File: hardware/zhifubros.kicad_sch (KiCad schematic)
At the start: 7 parts, among them J1 Conn_01x09, U1 XIAO-ESP32-C3-SMD, U2 GY-521, U3 GY-521

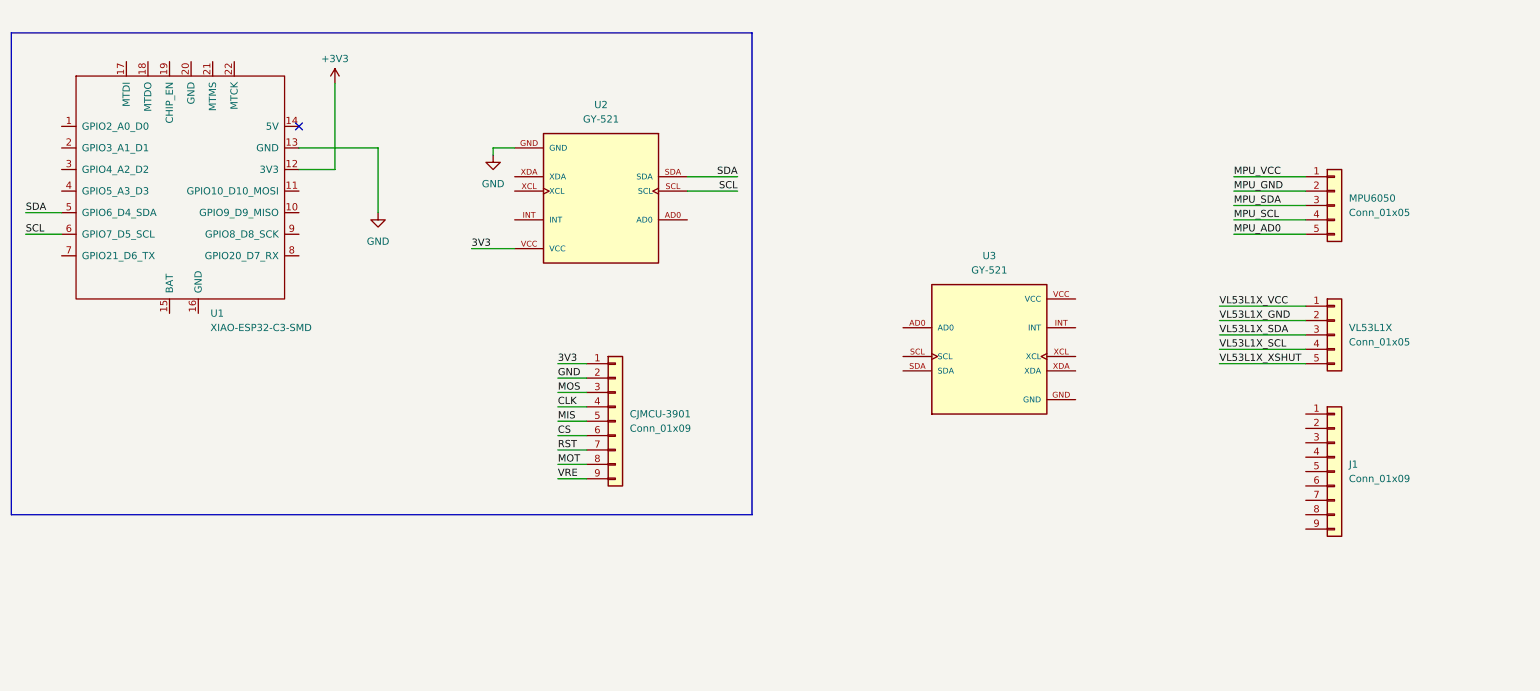
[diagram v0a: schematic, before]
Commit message: fix: schema
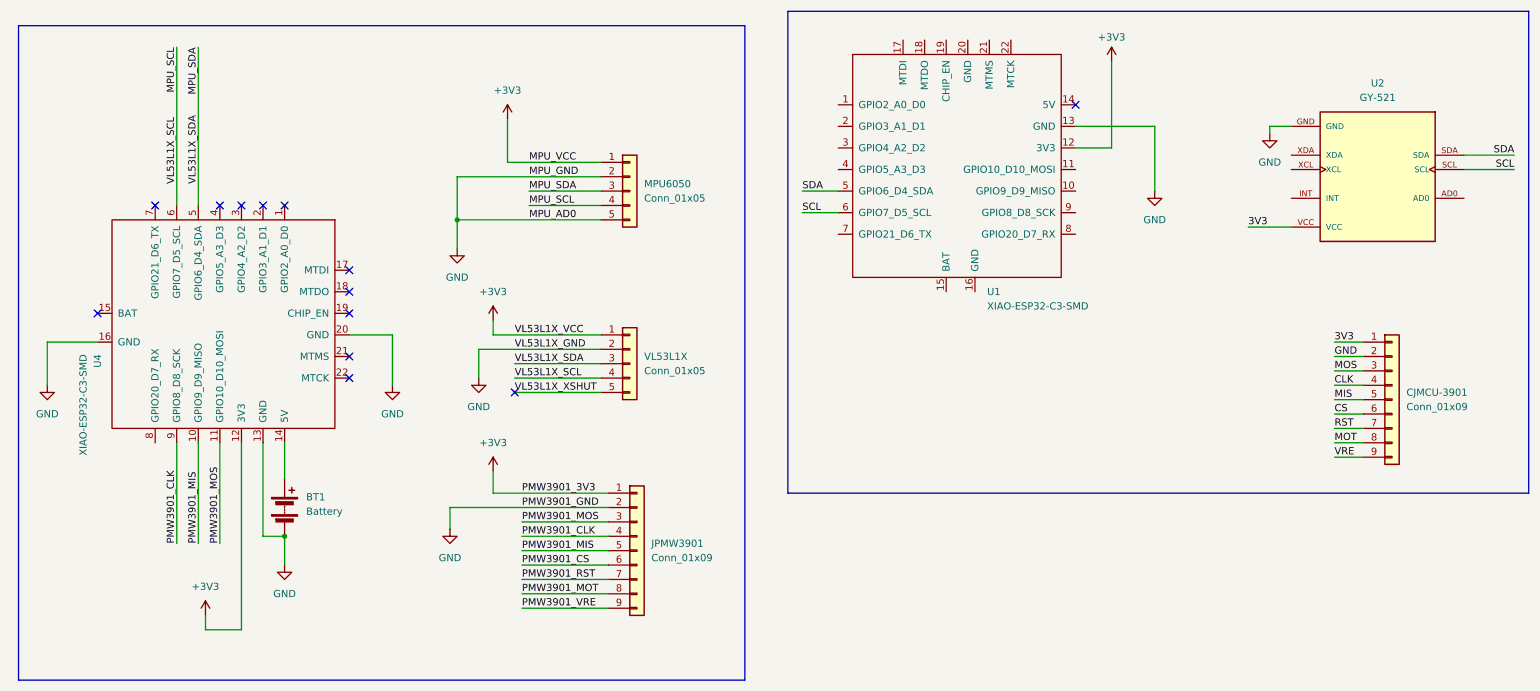
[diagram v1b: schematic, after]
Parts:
- removed U3: GY-521, GY-521:MODULE_GY-521, symbol mpu:GY-521
- added BT1: Battery, symbol Device:Battery
- added U4: XIAO-ESP32-C3-SMD, symbol xiao:XIAO-ESP32-C3-SMD
- renumbered J1 to JPMW3901
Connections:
- net MPU_AD0 is gone; now on net GND: MPU6050.5 (Pin_5)
- net MPU_GND is gone; now on net GND: MPU6050.2 (Pin_2)
- net MPU_VCC is gone; now on net +3V3: MPU6050.1 (Pin_1)
- net VL53L1X_GND is gone; now on net GND: VL53L1X.2 (Pin_2)
- net VL53L1X_SCL is gone; now on net MPU_SCL: VL53L1X.4 (Pin_4)
- net VL53L1X_SDA is gone; now on net MPU_SDA: VL53L1X.3 (Pin_3)
- net VL53L1X_VCC is gone; now on net +3V3: VL53L1X.1 (Pin_1)
- net +3V3: now also JPMW3901.1 (Pin_1), U4.12 (3V3)
- net GND: now also JPMW3901.2 (Pin_2), BT1.2 (-), U4.13 (GND), U4.16 (GND), U4.20 (GND)
- net MPU_SCL: now also U4.6 (GPIO7_D5_SCL)
- net MPU_SDA: now also U4.5 (GPIO6_D4_SDA)
- net PMW3901_MOS: now reaches JPMW3901.3 (Pin_3)
- net PMW3901_MOS: now also U4.11 (GPIO10_D10_MOSI)
- net PMW3901_CLK: now reaches JPMW3901.4 (Pin_4)
- net PMW3901_CLK: now also U4.9 (GPIO8_D8_SCK)
- net PMW3901_MIS: now reaches JPMW3901.5 (Pin_5)
- net PMW3901_MIS: now also U4.10 (GPIO9_D9_MISO)
- net PMW3901_CS: now reaches JPMW3901.6 (Pin_6)
- net PMW3901_RST: now reaches JPMW3901.7 (Pin_7)
- net PMW3901_MOT: now reaches JPMW3901.8 (Pin_8)
- net PMW3901_VRE: now reaches JPMW3901.9 (Pin_9)
- new net: BT1.1 (+), U4.14 (5V)
- no-connect marks 1 -> 13
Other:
- moved on the sheet: CJMCU-3901, JPMW3901, MPU6050, U1, U2, VL53L1X
